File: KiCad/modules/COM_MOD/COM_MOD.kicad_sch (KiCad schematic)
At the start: 31 parts, among them J1 Conn_01x01_Pin, J10 XF2J-1824-12A, J11 Conn_01x01_Pin, J12 Conn_01x01_Pin, J13 Conn_01x01_Pin, J14 Conn_01x01_Pin, J15 Conn_01x01_Pin, J16 Conn_01x01_Pin, J17 Conn_01x01_Pin, J18 Conn_01x01_Pin, J19 Conn_01x01_Pin, J2 Conn_01x01_Pin, J20 Conn_01x01_Pin, J21 Conn_01x01_Pin, J22 Conn_01x01_Pin, J23 Conn_01x01_Pin, J24 Conn_01x01_Pin, J3 Conn_01x01_Pin, J4 XF2J-1824-12A, J5 Conn_01x01_Pin, J6 Conn_01x01_Pin, J7 Conn_01x01_Pin, J8 Conn_01x01_Pin, J9 Conn_01x01_Pin, U1 HC32L110C6UA, U2 74HC688

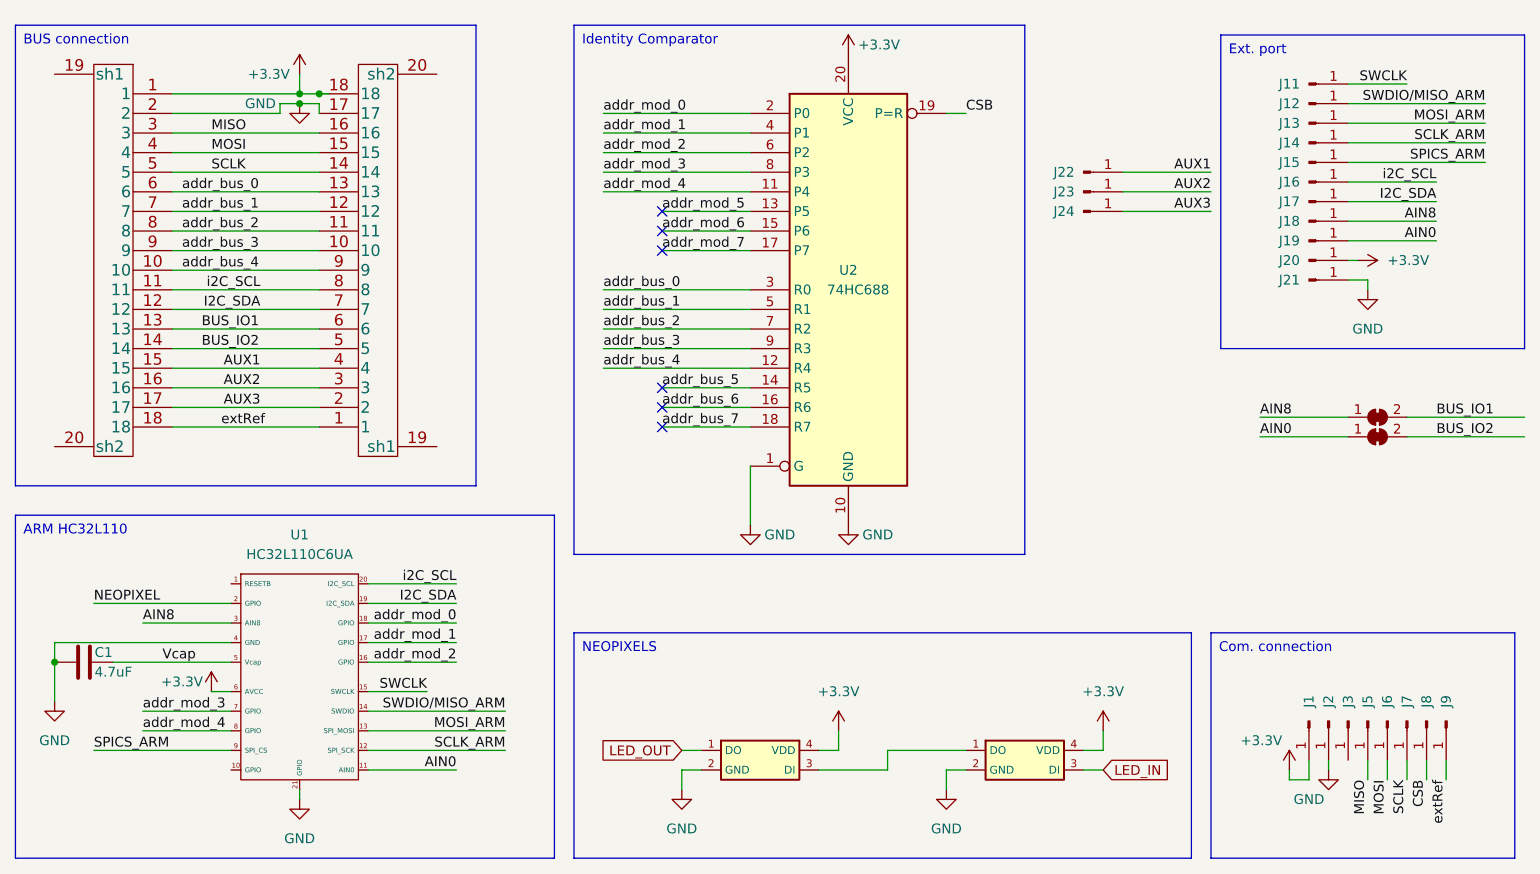
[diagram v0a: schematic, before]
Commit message: lot of updates on ads93,flex,commod,pad
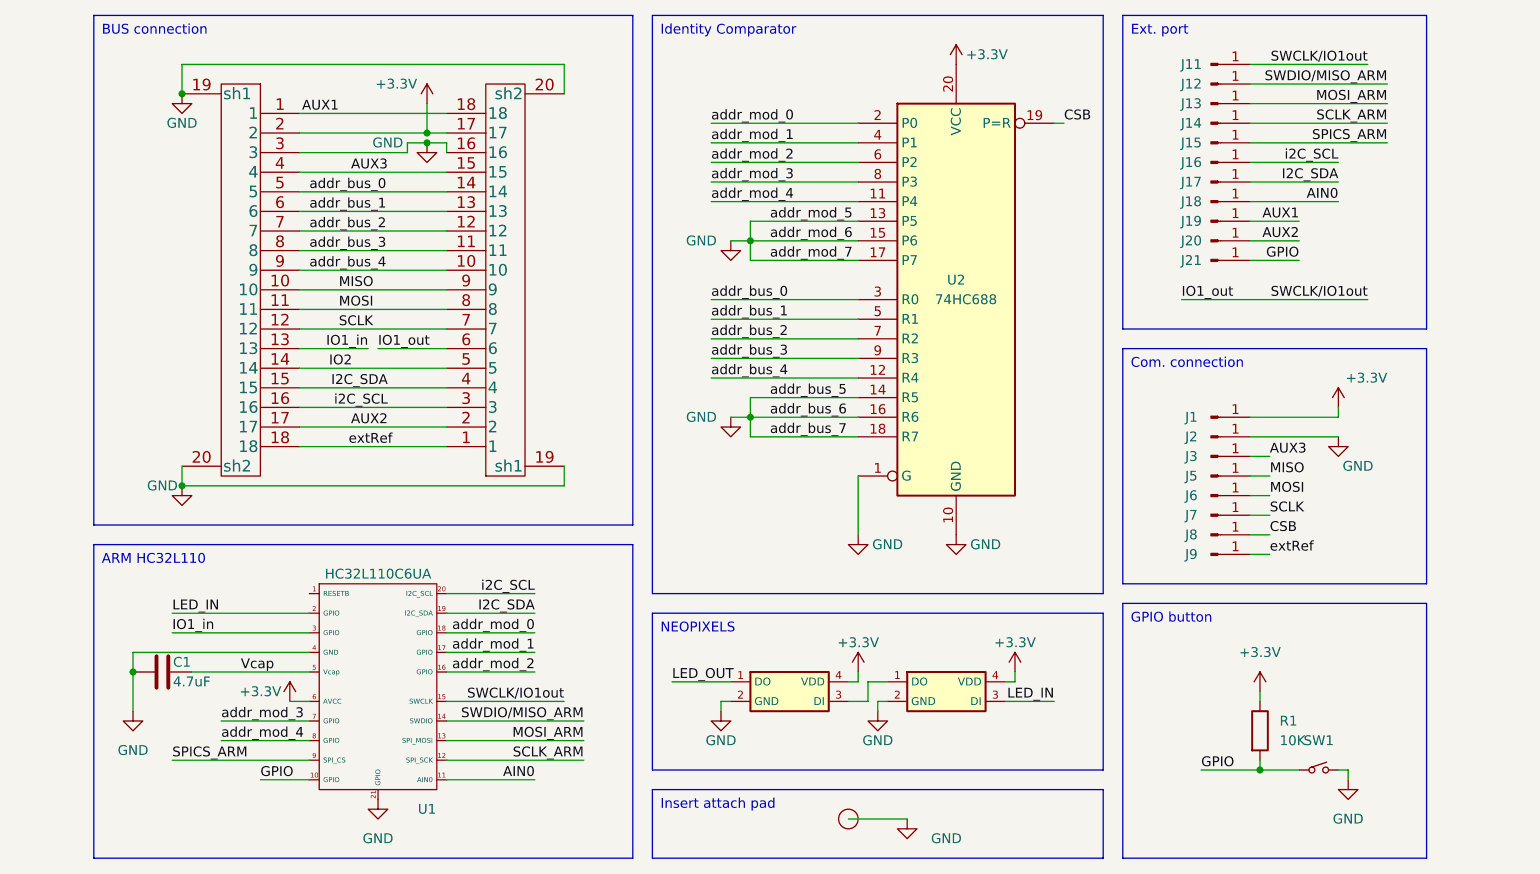
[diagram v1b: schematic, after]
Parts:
- removed J22, J23, J24: Conn_01x01_Pin, Connector_PinHeader_1.27mm:PinHeader_1x01_P1.27mm_Vertical, symbol Connector:Conn_01x01_Pin
- removed JP1, JP2: SolderJumper_2_Bridged, Jumper:SolderJumper-2_P1.3mm_Bridged_RoundedPad1.0x1.5mm, symbol Jumper:SolderJumper_2_Bridged
- added I1: smd_insert, 00_Custom:insert_1.2mm, symbol 00_custom:smd_insert
- added R1: 10K, Resistor_SMD:R_0402_1005Metric, symbol Device:R
- added SW1: NA, 00_Custom:SW-SMD_L3.9-W3.0-P4.45, symbol 00_custom:switch
- C1: LCSC (none) -> C23733
- J10, J4: footprint 00_custom-footprints:XUNPU_FPC_05F_18P_H20 -> 00_Custom:XUNPU_FPC_05F_18P_H20; symbol XF2J-1824-12A:XF2J-1824-12A -> 00_custom:XF2J-1824-12A; LCSC (none) -> C2856802
- LED1, LED2: footprint 00_custom-footprints:WS2812-2020 -> 00_Custom:WS2812-2020; symbol custom:WS2812-2020 -> 00_custom:WS2812-2020
- U1: footprint 00_custom-footprints:QFN-20-1EP_3x3mm_P0.4mm_EP1.4x1.4mm -> 00_Custom:QFN-20-1EP_3x3mm_P0.4mm_EP1.4x1.4mm; symbol XHSC:HC32L110C6UA -> 00_custom:HC32L110C6UA; LCSC (none) -> C493490
- U2: LCSC (none) -> C132045
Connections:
- net NEOPIXEL is gone; now on net LED_IN: U1.2 (P01)
- net SWCLK is gone; now on net IO1_out: J11.1 (Pin_1), U1.15 (P31)
- net addr_bus_5 is gone; now on net GND: U2.14 (R5)
- net addr_bus_6 is gone; now on net GND: U2.16 (R6)
- net addr_bus_7 is gone; now on net GND: U2.18 (R7)
- net addr_mod_5 is gone; now on net GND: U2.13 (P5)
- net addr_mod_6 is gone; now on net GND: U2.15 (P6)
- net addr_mod_7 is gone; now on net GND: U2.17 (P7)
- net +3.3V: now also J10.17, J4.2, R1.1; no longer J10.18, J20.1 (Pin_1), J4.1
- net AIN0: now also J18.1 (Pin_1); no longer J19.1 (Pin_1)
- net AUX1: now also J10.18, J19.1 (Pin_1), J4.1; no longer J10.4, J4.15
- net AUX2: now also J10.2, J20.1 (Pin_1), J4.17; no longer J10.3, J4.16
- net AUX3: now also J10.15, J3.1 (Pin_1), J4.4; no longer J10.2, J4.17
- net GND: now also J10.16, J10.19 (sh1), J10.20 (sh2), J4.19 (sh1), J4.20 (sh2), J4.3, I1.1 (conn), SW1.2; no longer J10.17, J21.1 (Pin_1), J4.2
- net I2C_SDA: now also J10.4, J4.15; no longer J10.7, J4.12
- net MISO: now also J10.9, J4.10; no longer J10.16, J4.3
- net MOSI: now also J10.8, J4.11; no longer J10.15, J4.4
- net SCLK: now also J10.7, J4.12; no longer J10.14, J4.5
- net addr_bus_0: now also J10.14, J4.5; no longer J10.13, J4.6
- net addr_bus_1: now also J10.13, J4.6; no longer J10.12, J4.7
- net addr_bus_2: now also J10.12, J4.7; no longer J10.11, J4.8
- net addr_bus_3: now also J10.11, J4.8; no longer J10.10, J4.9
- net addr_bus_4: now also J10.10, J4.9; no longer J10.9, J4.10
- net i2C_SCL: now also J10.3, J4.16; no longer J10.8, J4.11
- net GPIO: now reaches U1.10 (P23)
- net GPIO: now also J21.1 (Pin_1), R1.2, SW1.1
- net AIN8 renamed IO1_in
- net IO1_in: now also J4.13; no longer J18.1 (Pin_1)
- net BUS_IO1 renamed IO1_out
- net IO1_out: no longer J4.13
- net BUS_IO2 renamed IO2
- no-connect marks 6 -> 0
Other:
- company: (none) -> Aightech
- title: (none) -> CleverHand Communication Module
- moved on the sheet: C1, J1, J11, J12, J13, J14, J15, J16, J17, J18, J2, J3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
